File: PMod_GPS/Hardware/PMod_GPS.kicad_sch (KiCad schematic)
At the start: 3 parts, among them J1 Conn_02x06_Odd_Even, U1 NEO-M8M

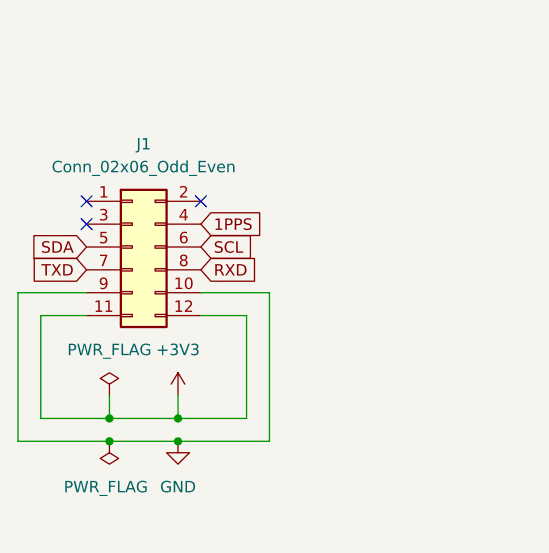
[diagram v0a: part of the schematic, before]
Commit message: correct the error for the RX and TX being the wrong way round #73 on schematic
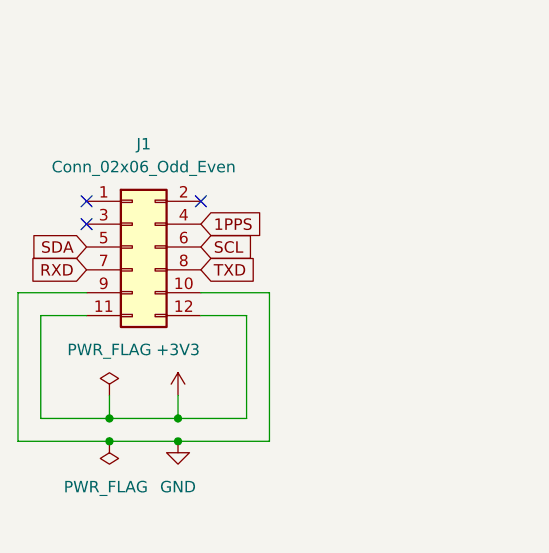
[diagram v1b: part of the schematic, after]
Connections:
- net RXD: now also J1.7 (Pin_7); no longer J1.8 (Pin_8)
- net TXD: now also J1.8 (Pin_8); no longer J1.7 (Pin_7)
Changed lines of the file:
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@@
     )
   )
-  (global_label "RXD" (shape input) (at 66.04 74.93 0) (fields_autoplaced)
-    (effects (font (size 1.27 1.27)) (justify left))
-    (property "Intersheet References" "${INTERSHEET_REFS}" (id 0) (at 72.2026 75.0094 0)
-      (effects (font (size 1.27 1.27)) (justify left) hide)
+  (global_label "RXD" (shape input) (at 53.34 74.93 180) (fields_autoplaced)
+    (effects (font (size 1.27 1.27)) (justify right))
+    (property "Intersheet References" "${INTERSHEET_REFS}" (id 0) (at 47.1774 74.8506 0)
+      (effects (font (size 1.27 1.27)) (justify right) hide)
     )
   )
@@
     )
   )
-  (global_label "TXD" (shape input) (at 53.34 74.93 180) (fields_autoplaced)
-    (effects (font (size 1.27 1.27)) (justify right))
-    (property "Intersheet References" "${INTERSHEET_REFS}" (id 0) (at 47.4798 74.8506 0)
-      (effects (font (size 1.27 1.27)) (justify right) hide)
+  (global_label "TXD" (shape input) (at 66.04 74.93 0) (fields_autoplaced)
+    (effects (font (size 1.27 1.27)) (justify left))
+    (property "Intersheet References" "${INTERSHEET_REFS}" (id 0) (at 71.9002 75.0094 0)
+      (effects (font (size 1.27 1.27)) (justify left) hide)
     )
   )
